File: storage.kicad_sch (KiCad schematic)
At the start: 9 parts, among them J4 503398-1892, J5 2171840001

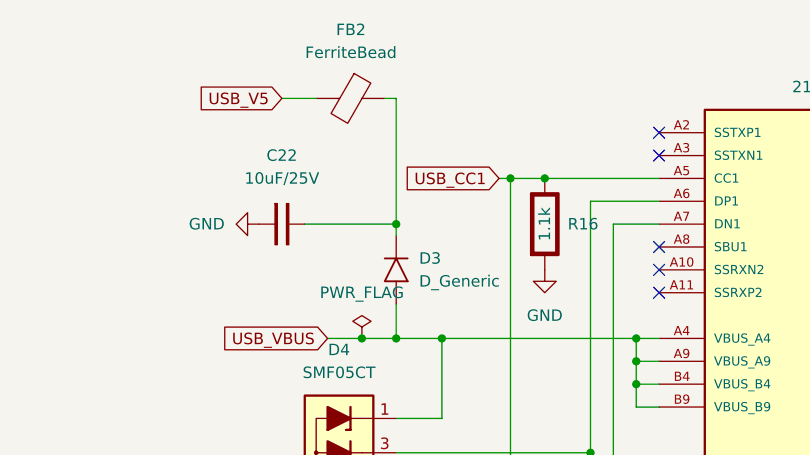
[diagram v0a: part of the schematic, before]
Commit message: pcb / inital work
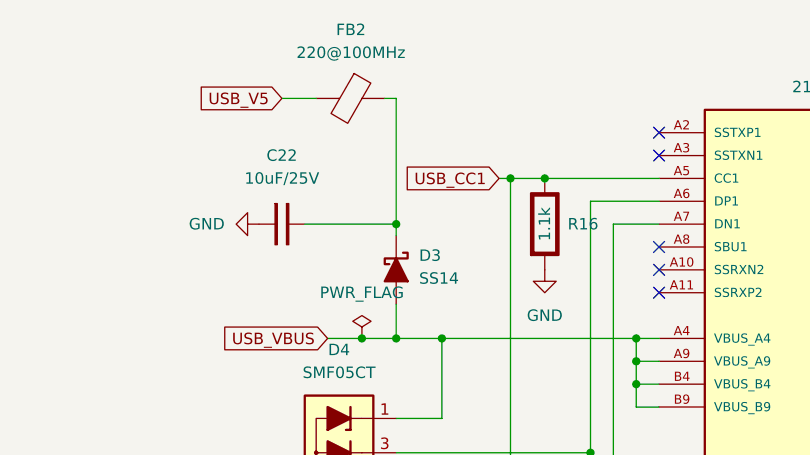
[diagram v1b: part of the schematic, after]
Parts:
- removed D3: D_Generic, symbol PCM_4ms_Diode:D_Generic
- added D3: SS14, PCM_Diode_SMD_AKL:D_SMA, symbol PCM_Diode_Schottky_AKL:SS14
- C22: footprint Capacitor_THT:C_Disc_D3.0mm_W2.0mm_P2.50mm -> Capacitor_SMD:C_0805_2012Metric
- FB2: value FerriteBead -> 220@100MHz; footprint (none) -> PCM_Ferrite_SMD_AKL:Ferrite_0603_1608Metric
- J4: footprint 503398-1892:MOLEX_503398-1892 -> uwu:MOLEX_503398-1892
- J5: footprint 2171840001:MOLEX_2171840001 -> uwu:MOLEX_2171840001
- R16, R17, R36: footprint (none) -> Resistor_SMD:R_0603_1608Metric
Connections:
- net USB_VBUS: now also D3.2 (A)
- net at C22.2, FB2.1: now also D3.1 (K)
